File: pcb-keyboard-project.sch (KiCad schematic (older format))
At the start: 24 parts, among them SW1 SW_PUSH, U1 ATmega32U4-AU, Y1 16MHz

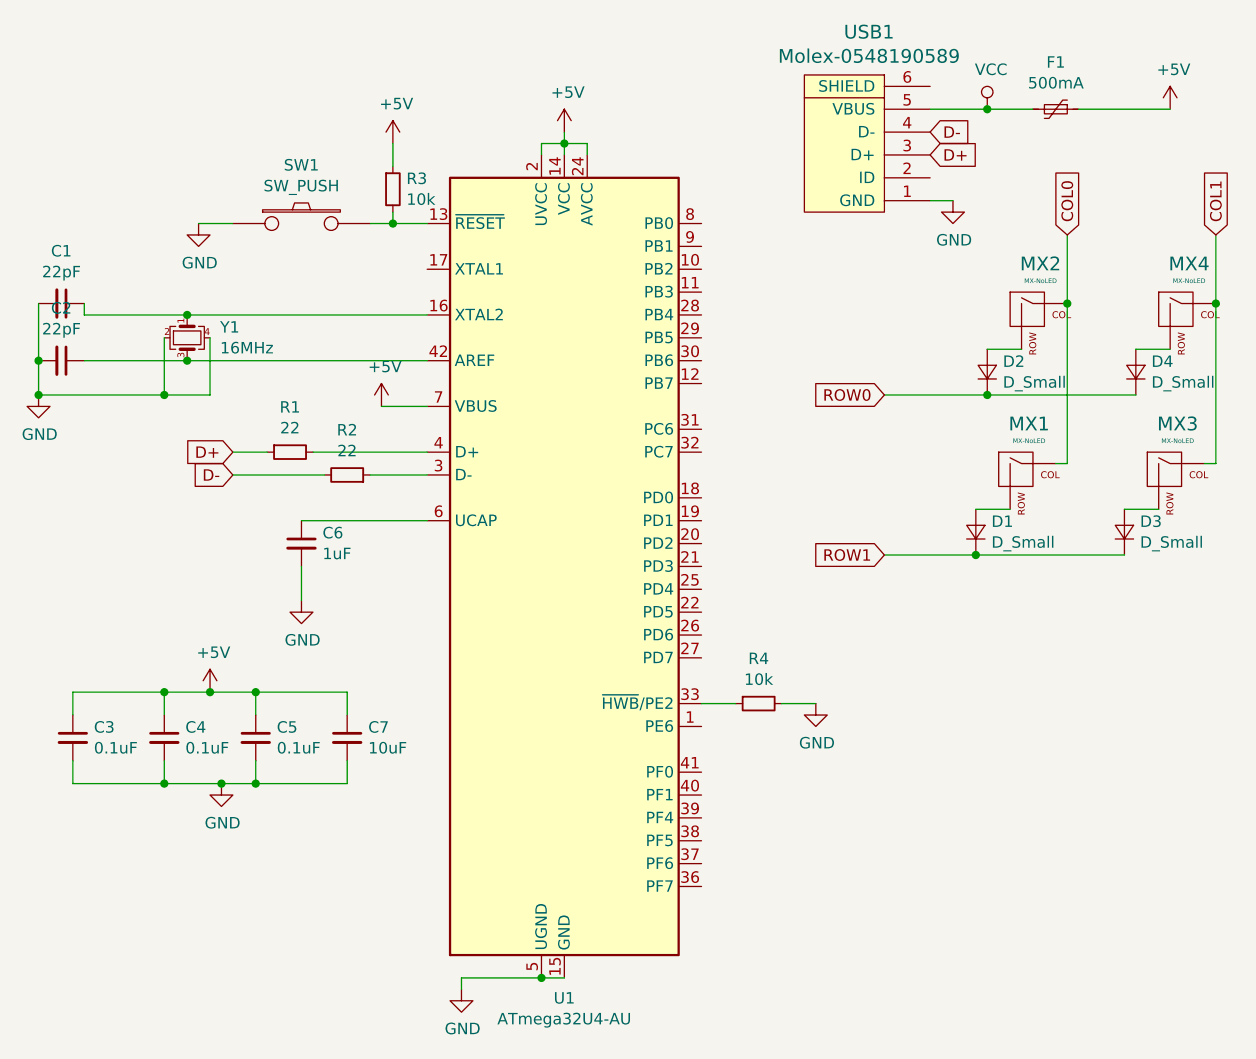
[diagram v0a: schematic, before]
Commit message: pcb finish
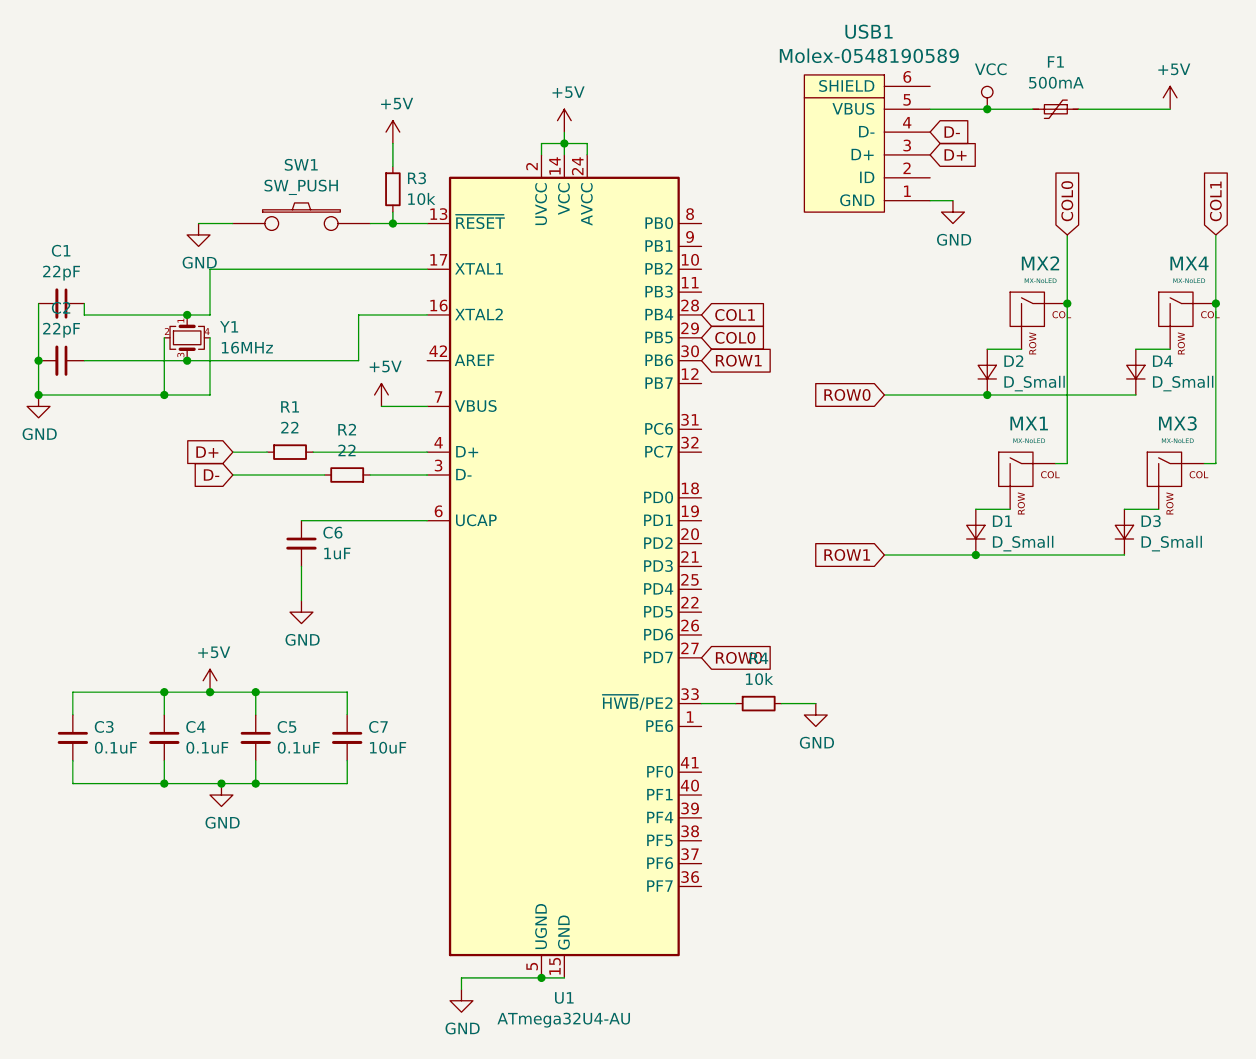
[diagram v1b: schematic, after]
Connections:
- net COL0: now also U1.29 (PB5)
- net COL1: now also U1.28 (PB4)
- net ROW0: now also U1.27 (PD7)
- net ROW1: now also U1.30 (PB6)
- net at C1.1, Y1.1: now also U1.17 (XTAL1); no longer U1.16 (XTAL2)
- net at C2.1, Y1.3: now also U1.16 (XTAL2); no longer U1.42 (AREF)
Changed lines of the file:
@@
 $EndComp
 Wire Wire Line
-	2850 2400 1800 2400
-Wire Wire Line
-	1800 2600 2850 2600
+	1800 2600 2550 2600
 $Comp
 L Device:C_Small C1
@@
 Wire Wire Line
 	1350 2400 1350 2350
-Connection ~ 1800 2400
 Wire Wire Line
 	1150 2350 1150 2600
@@
 Text GLabel 4850 3450 0    50   Input ~ 0
 ROW1
+Wire Wire Line
+	2850 2200 1900 2200
+Wire Wire Line
+	1900 2200 1900 2400
+Wire Wire Line
+	1900 2400 1800 2400
+Connection ~ 1800 2400
+Wire Wire Line
+	2550 2600 2550 2400
+Wire Wire Line
+	2550 2400 2850 2400
+Text GLabel 4050 3900 2    50   Input ~ 0
+ROW0
+Text GLabel 4050 2600 2    50   Input ~ 0
+ROW1
+Text GLabel 4050 2500 2    50   Input ~ 0
+COL0
+Text GLabel 4050 2400 2    50   Input ~ 0
+COL1
 $EndSCHEMATC
